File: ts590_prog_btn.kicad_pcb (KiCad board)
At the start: 2 copper layers, 18 parts, among them J1 DB9, SW1 PTT, SW2 PF2, SW3 PF4, SW4 PF1, SW5 PF3, SW6 UP, SW7 DOWN, SW8 MIC_EXT_PWR, SW9 PTT_LOCK

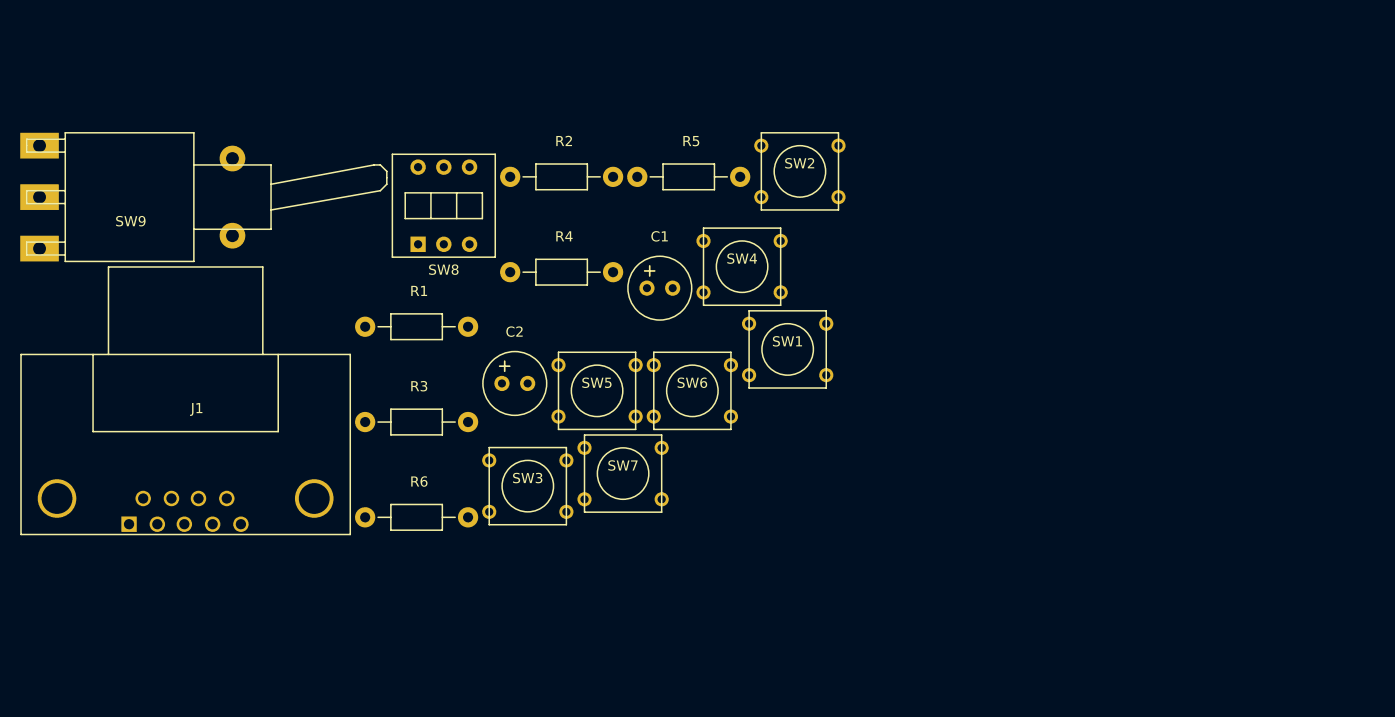
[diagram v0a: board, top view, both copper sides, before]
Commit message: added the first pcb draw
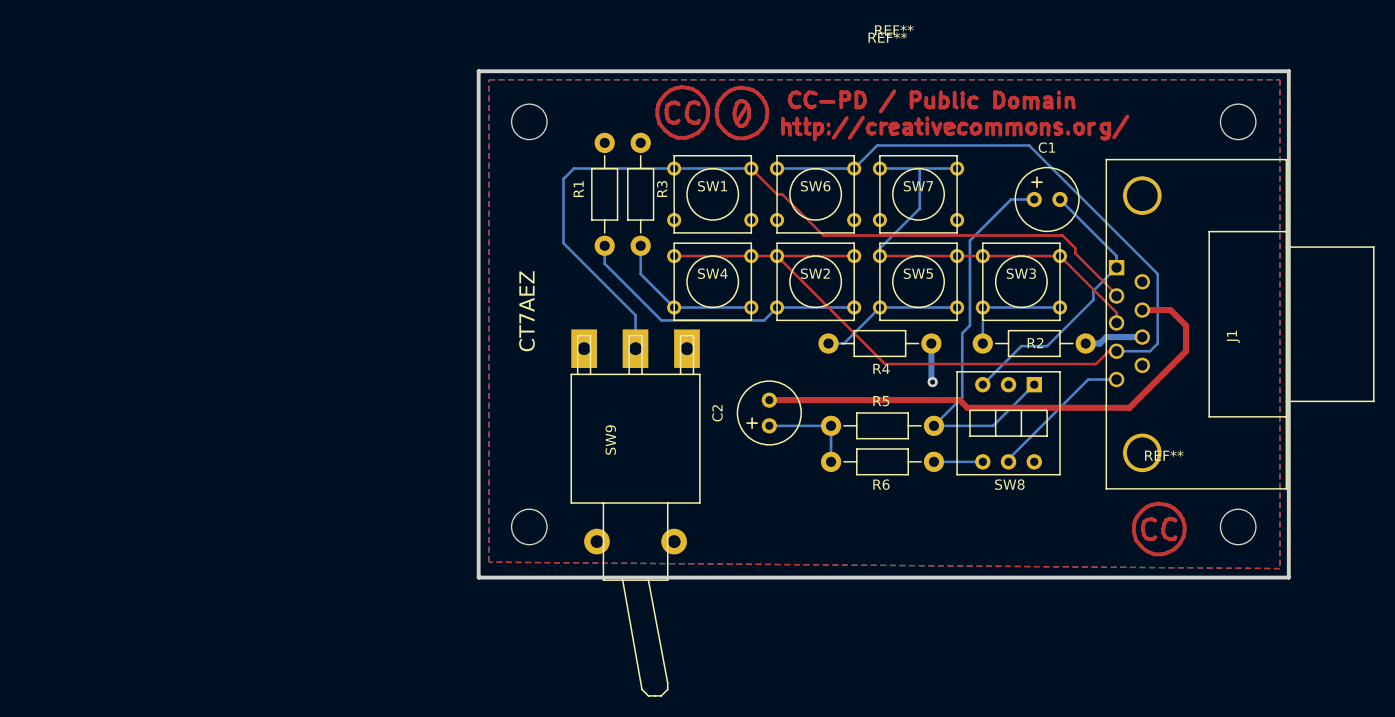
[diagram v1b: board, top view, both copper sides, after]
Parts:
- added REF**: EuroBoard_viertel_Type-I_80mmX50mm_holes, EuroBoard_Outline:EuroBoard_viertel_Type-I_80mmX50mm_holes, F.Cu at (109.5, 99.3)
- added REF**: Symbol_CreativeCommons_CopperTop_Type2_Small, Symbols:Symbol_CreativeCommons_CopperTop_Type2_Small, F.Cu at (176.5, 94.6)
- added REF**: Symbol_CreativeCommonsPublicDomain_CopperTop_Small, Symbols:Symbol_CreativeCommonsPublicDomain_CopperTop_Small, F.Cu at (149.2, 53.3)
- moved J1 95.2 mm to (173.7, 74.2), turned to 270 degrees
- moved SW9 60.7 mm to (125.0, 76.7), turned to 270 degrees
- moved SW8 59.8 mm to (161.8, 84.1), turned to 180 degrees
- moved SW3 52.8 mm to (163.1, 70.1)
- moved R2 49.5 mm to (164.3, 76.2)
- moved R6 46.3 mm to (149.4, 87.9), turned to 180 degrees
- moved SW7 40.1 mm to (152.9, 61.5)
- moved C1 39.2 mm to (164.3, 62.0)
- moved SW5 33.5 mm to (152.9, 70.1)
- moved R4 32.2 mm to (149.1, 76.2)
- moved R3 31.5 mm to (125.5, 61.5), turned to 90 degrees
- moved R5 31.2 mm to (149.4, 84.3)
- moved C2 26.7 mm to (138.2, 84.3), turned to 90 degrees
- moved SW6 22.9 mm to (142.7, 61.5)
- moved R1 22.7 mm to (121.9, 61.5), turned to 90 degrees
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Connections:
- J1 pad 6: Net-(J1-Pad6) -> (no net)
- J1 pad 9: Net-(J1-Pad9) -> (no net)
- SW8 pad 2: /EXTMIC -> (no net)
- SW8 pad 6: Net-(SW8-Pad6) -> (no net)
- SW9 pad 1: Net-(SW9-Pad1) -> (no net)
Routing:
- net /MICCN4_UP: track 0.00 -> 111.3 mm
- net /MICCN2_PTT: track 0.00 -> 80.3 mm
- net GNDA: track 0.00 -> 51.3 mm
- net /MICCN3_DOWN: track 0.00 -> 44.8 mm
- net /MIC_ELECT: track 0.00 -> 39.4 mm
- net Net-(R1-Pad1): track 0.00 -> 29.3 mm
- net /MICCN1_MIC: track 0.00 -> 27.6 mm
- net Net-(R3-Pad1): track 0.00 -> 15.1 mm
- net /MICCN5_8V: track 0.00 -> 14.2 mm
- net Net-(R4-Pad1): track 0.00 -> 14.2 mm
- net Net-(R2-Pad1): track 0.00 -> 11.2 mm
- net GND: track 0.00 -> 9.71 mm, vias 0 -> 1
- net Net-(C2-Pad1): track 0.00 -> 9.65 mm
- net /MICCN5_8V_PWRSW: track 0.00 -> 4.83 mm
- added copper zone on F.Cu, net GND
- added copper zone on B.Cu, net GNDA
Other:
- board outline added: 80 x 50 mm
- net class Default: trace_width 0.25 -> 0.254; via_dia 0.6 -> 1; via_drill 0.4 -> 0.5
- net class PWR added: clearance 0.2, trace_width 0.6, via_dia 1, via_drill 0.5
- board text added: "CT7AEZ"
- board text added: "Este trabalho está licenciado sob uma Licença Creative Commons Atribuição 4.0 Internacional. Para ver uma cópia desta licença, visite http://creativecommons.org/licenses/by/4.0/."
